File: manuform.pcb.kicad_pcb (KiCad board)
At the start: 2 copper layers, 90 x 90.5 mm, 55 parts, among them J1 Conn_01x05, J3 Conn_01x01, J4 Conn_01x01, SW1 SW_DIP_x01, SW2 SW_DIP_x01, SW3 SW_DIP_x01, SW4 SW_DIP_x01

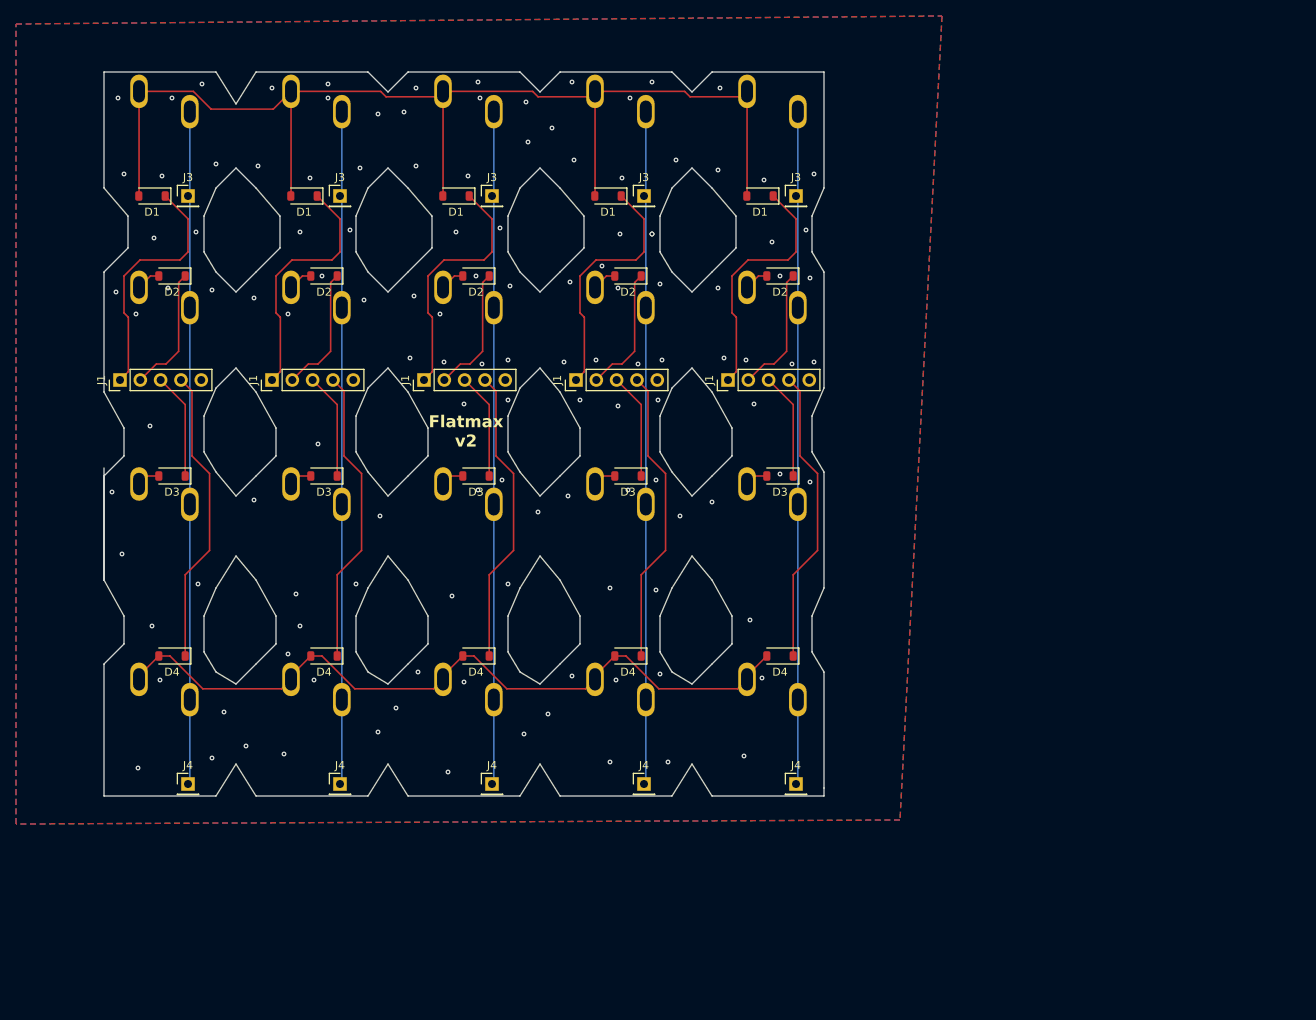
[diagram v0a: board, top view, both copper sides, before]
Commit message: kalih choc v2 flex PCB
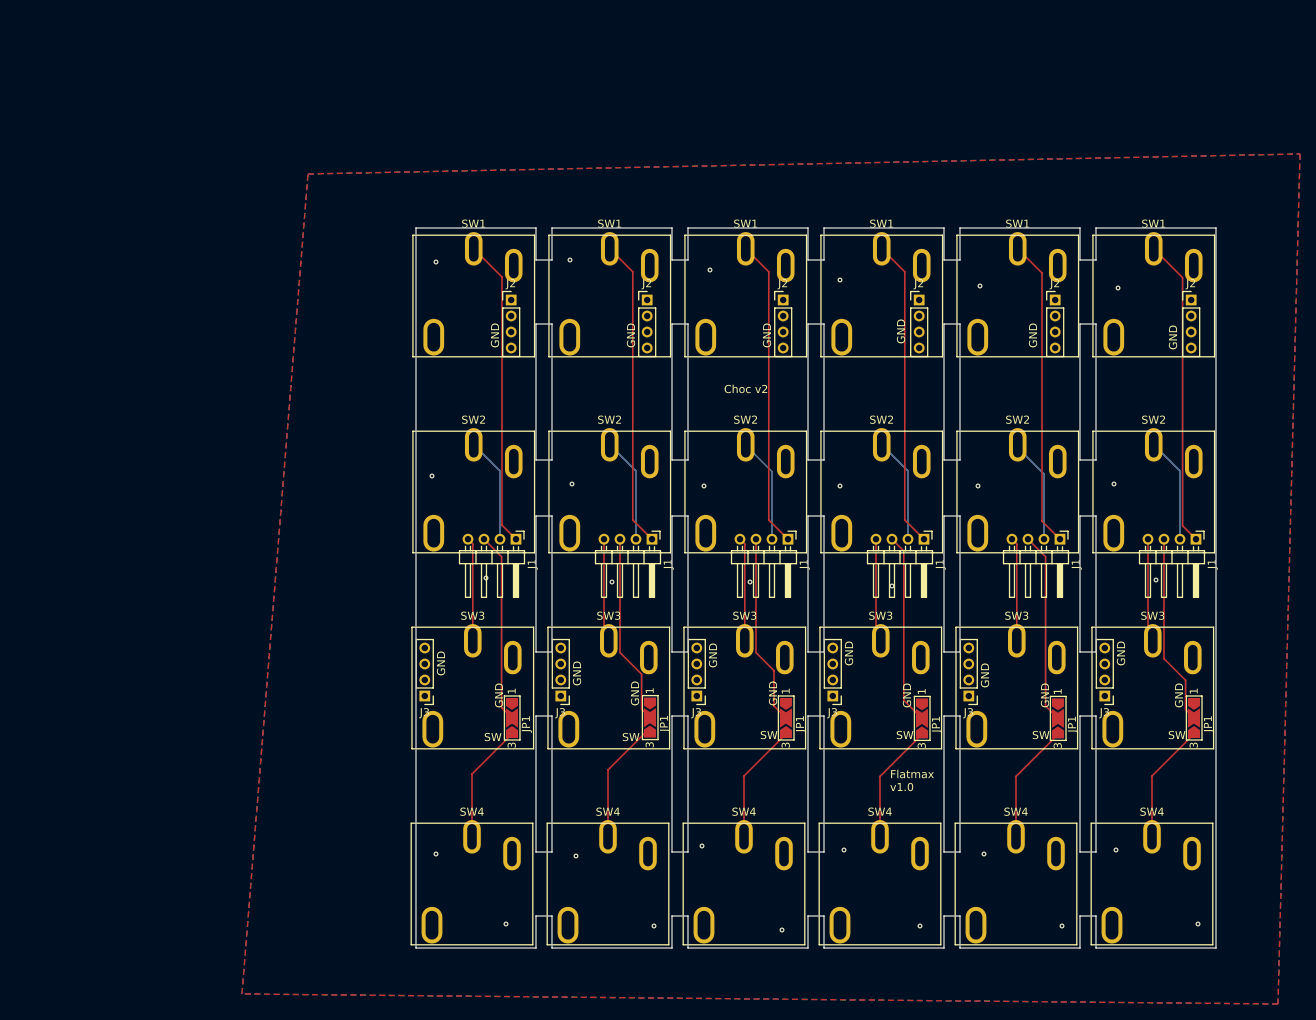
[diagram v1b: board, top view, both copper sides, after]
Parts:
- removed D1 (x5), D2 (x5), D3 (x5), D4 (x5): D, Diode_SMD:D_SOD-123
- removed the J1 at (117.0, 56.0)
- removed the J1 at (193.0, 56.0)
- removed the J1 at (155.0, 56.0)
- removed the J1 at (136.0, 56.0)
- removed the J1 at (174.0, 56.0)
- removed the J3 at (125.5, 33.0)
- removed the J3 at (163.5, 33.0)
- removed the J3 at (182.5, 33.0)
- removed the J3 at (144.5, 33.0)
- removed the J3 at (201.5, 33.0)
- removed J4 (x5): Conn_01x01, Connector_PinHeader_2.54mm:PinHeader_1x01_P2.54mm_Vertical
- removed the SW1 at (119.4, 19.9)
- removed the SW1 at (176.4, 19.9)
- removed the SW1 at (157.4, 19.9)
- removed the SW1 at (138.4, 19.9)
- removed the SW1 at (195.4, 19.9)
- removed the SW2 at (119.4, 44.4)
- removed the SW2 at (157.4, 44.4)
- removed the SW2 at (195.4, 44.4)
- removed the SW2 at (176.4, 44.4)
- removed the SW2 at (138.4, 44.4)
- removed the SW3 at (138.4, 69.0)
- removed the SW3 at (195.4, 69.0)
- removed the SW3 at (119.4, 69.0)
- removed the SW3 at (176.4, 69.0)
- removed the SW3 at (157.4, 69.0)
- removed the SW4 at (119.4, 93.4)
- removed the SW4 at (157.4, 93.4)
- removed the SW4 at (138.4, 93.4)
- removed the SW4 at (195.4, 93.4)
- removed the SW4 at (176.4, 93.4)
- added J1: Conn_01x04, Connector_PinHeader_2.00mm:PinHeader_1x04_P2.00mm_Horizontal, F.Cu at (183.5, 75.9)
- added J1: Conn_01x04, Connector_PinHeader_2.00mm:PinHeader_1x04_P2.00mm_Horizontal, F.Cu at (217.5, 75.9)
- added J1: Conn_01x04, Connector_PinHeader_2.00mm:PinHeader_1x04_P2.00mm_Horizontal, F.Cu at (234.5, 75.9)
- added J1: Conn_01x04, Connector_PinHeader_2.00mm:PinHeader_1x04_P2.00mm_Horizontal, F.Cu at (251.5, 75.9)
- added J1: Conn_01x04, Connector_PinHeader_2.00mm:PinHeader_1x04_P2.00mm_Horizontal, F.Cu at (166.5, 75.9)
- added J1: Conn_01x04, Connector_PinHeader_2.00mm:PinHeader_1x04_P2.00mm_Horizontal, F.Cu at (200.5, 75.9)
- added J2: Conn_01x04, Connector_PinHeader_2.00mm:PinHeader_1x04_P2.00mm_Vertical, F.Cu at (216.9, 46.0)
- added J2: Conn_01x04, Connector_PinHeader_2.00mm:PinHeader_1x04_P2.00mm_Vertical, F.Cu at (250.9, 46.0)
- added J2: Conn_01x04, Connector_PinHeader_2.00mm:PinHeader_1x04_P2.00mm_Vertical, F.Cu at (182.9, 46.0)
- added J2: Conn_01x04, Connector_PinHeader_2.00mm:PinHeader_1x04_P2.00mm_Vertical, F.Cu at (165.9, 46.0)
- added J2: Conn_01x04, Connector_PinHeader_2.00mm:PinHeader_1x04_P2.00mm_Vertical, F.Cu at (233.9, 46.0)
- added J2: Conn_01x04, Connector_PinHeader_2.00mm:PinHeader_1x04_P2.00mm_Vertical, F.Cu at (199.9, 46.0)
- added J3: Conn_01x04, Connector_PinHeader_2.00mm:PinHeader_1x04_P2.00mm_Vertical, F.Cu at (240.1, 95.5)
- added J3: Conn_01x04, Connector_PinHeader_2.00mm:PinHeader_1x04_P2.00mm_Vertical, F.Cu at (155.1, 95.5)
- added J3: Conn_01x04, Connector_PinHeader_2.00mm:PinHeader_1x04_P2.00mm_Vertical, F.Cu at (223.1, 95.5)
- added J3: Conn_01x04, Connector_PinHeader_2.00mm:PinHeader_1x04_P2.00mm_Vertical, F.Cu at (206.1, 95.5)
- added J3: Conn_01x04, Connector_PinHeader_2.00mm:PinHeader_1x04_P2.00mm_Vertical, F.Cu at (172.1, 95.5)
- added J3: Conn_01x04, Connector_PinHeader_2.00mm:PinHeader_1x04_P2.00mm_Vertical, F.Cu at (189.1, 95.5)
- added JP1: SolderJumper_3_Open, Jumper:SolderJumper-3_P2.0mm_Open_TrianglePad1.0x1.5mm_NumberLabels, F.Cu at (251.2, 98.2)
- added JP1: SolderJumper_3_Open, Jumper:SolderJumper-3_P2.0mm_Open_TrianglePad1.0x1.5mm_NumberLabels, F.Cu at (217.2, 98.3)
- added JP1: SolderJumper_3_Open, Jumper:SolderJumper-3_P2.0mm_Open_TrianglePad1.0x1.5mm_NumberLabels, F.Cu at (166.0, 98.2)
- added JP1: SolderJumper_3_Open, Jumper:SolderJumper-3_P2.0mm_Open_TrianglePad1.0x1.5mm_NumberLabels, F.Cu at (234.2, 98.3)
- added JP1: SolderJumper_3_Open, Jumper:SolderJumper-3_P2.0mm_Open_TrianglePad1.0x1.5mm_NumberLabels, F.Cu at (200.2, 98.2)
- added JP1: SolderJumper_3_Open, Jumper:SolderJumper-3_P2.0mm_Open_TrianglePad1.0x1.5mm_NumberLabels, F.Cu at (183.2, 98.2)
- added SW1: SW_DIP_x01, switchCustom:SW_Kailh_Choc_V2_elongated, F.Cu at (246.2, 45.5)
- added SW1: SW_DIP_x01, switchCustom:SW_Kailh_Choc_V2_elongated, F.Cu at (229.2, 45.5)
- added SW1: SW_DIP_x01, switchCustom:SW_Kailh_Choc_V2_elongated, F.Cu at (195.2, 45.5)
- added SW1: SW_DIP_x01, switchCustom:SW_Kailh_Choc_V2_elongated, F.Cu at (161.2, 45.5)
- added SW1: SW_DIP_x01, switchCustom:SW_Kailh_Choc_V2_elongated, F.Cu at (178.2, 45.5)
- added SW1: SW_DIP_x01, switchCustom:SW_Kailh_Choc_V2_elongated, F.Cu at (212.2, 45.5)
- added SW2: SW_DIP_x01, switchCustom:SW_Kailh_Choc_V2_elongated, F.Cu at (195.2, 70.0)
- added SW2: SW_DIP_x01, switchCustom:SW_Kailh_Choc_V2_elongated, F.Cu at (246.2, 70.0)
- added SW2: SW_DIP_x01, switchCustom:SW_Kailh_Choc_V2_elongated, F.Cu at (178.2, 70.0)
- added SW2: SW_DIP_x01, switchCustom:SW_Kailh_Choc_V2_elongated, F.Cu at (229.2, 70.0)
- added SW2: SW_DIP_x01, switchCustom:SW_Kailh_Choc_V2_elongated, F.Cu at (161.2, 70.0)
- added SW2: SW_DIP_x01, switchCustom:SW_Kailh_Choc_V2_elongated, F.Cu at (212.2, 70.0)
- added SW3: SW_DIP_x01, switchCustom:SW_Kailh_Choc_V2_elongated, F.Cu at (178.1, 94.5)
- added SW3: SW_DIP_x01, switchCustom:SW_Kailh_Choc_V2_elongated, F.Cu at (229.1, 94.5)
- added SW3: SW_DIP_x01, switchCustom:SW_Kailh_Choc_V2_elongated, F.Cu at (212.1, 94.5)
- added SW3: SW_DIP_x01, switchCustom:SW_Kailh_Choc_V2_elongated, F.Cu at (195.1, 94.5)
- added SW3: SW_DIP_x01, switchCustom:SW_Kailh_Choc_V2_elongated, F.Cu at (161.1, 94.5)
- added SW3: SW_DIP_x01, switchCustom:SW_Kailh_Choc_V2_elongated, F.Cu at (246.1, 94.5)
- added SW4: SW_DIP_x01, switchCustom:SW_Kailh_Choc_V2_elongated, F.Cu at (178.0, 119.0)
- added SW4: SW_DIP_x01, switchCustom:SW_Kailh_Choc_V2_elongated, F.Cu at (161.0, 119.0)
- added SW4: SW_DIP_x01, switchCustom:SW_Kailh_Choc_V2_elongated, F.Cu at (212.0, 119.0)
- added SW4: SW_DIP_x01, switchCustom:SW_Kailh_Choc_V2_elongated, F.Cu at (246.0, 119.0)
- added SW4: SW_DIP_x01, switchCustom:SW_Kailh_Choc_V2_elongated, F.Cu at (229.0, 119.0)
- added SW4: SW_DIP_x01, switchCustom:SW_Kailh_Choc_V2_elongated, F.Cu at (195.0, 119.0)
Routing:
- net Net-(J3-Pin_1): track 420.7 -> 0.00 mm
- net Net-(J1-Pin_1): track 0.00 -> 230.9 mm
- net Net-(D4-K): track 186.2 -> 0.00 mm
- net Net-(D1-K): track 155.4 -> 0.00 mm
- net Net-(D1-A): track 145.0 -> 0.00 mm
- net Net-(J1-Pin_3): track 0.00 -> 143.4 mm
- net Net-(D4-A): track 94.6 -> 0.00 mm
- net Net-(JP1-B): track 0.00 -> 90.4 mm
- net Net-(D2-K): track 80.1 -> 0.00 mm
- net Net-(J1-Pin_2): track 0.00 -> 79.0 mm
- net Net-(J1-Pin_4): track 0.00 -> 77.7 mm
- net Net-(D3-K): track 66.4 -> 0.00 mm
- net Net-(D2-A): track 15.3 -> 0.00 mm
- net Net-(D3-A): track 14.4 -> 0.00 mm
- net GND: vias 128 -> 29
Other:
- board size 90 x 90.5 mm -> 100 x 90 mm
- board text added: "Choc v2"
- board text added: "Flatmax v1.0"
- board text added: "GND"
- board text added: "SW"
- board text removed: "Flatmax v2"
